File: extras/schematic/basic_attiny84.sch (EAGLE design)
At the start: 14 parts, among them U1 SI4703

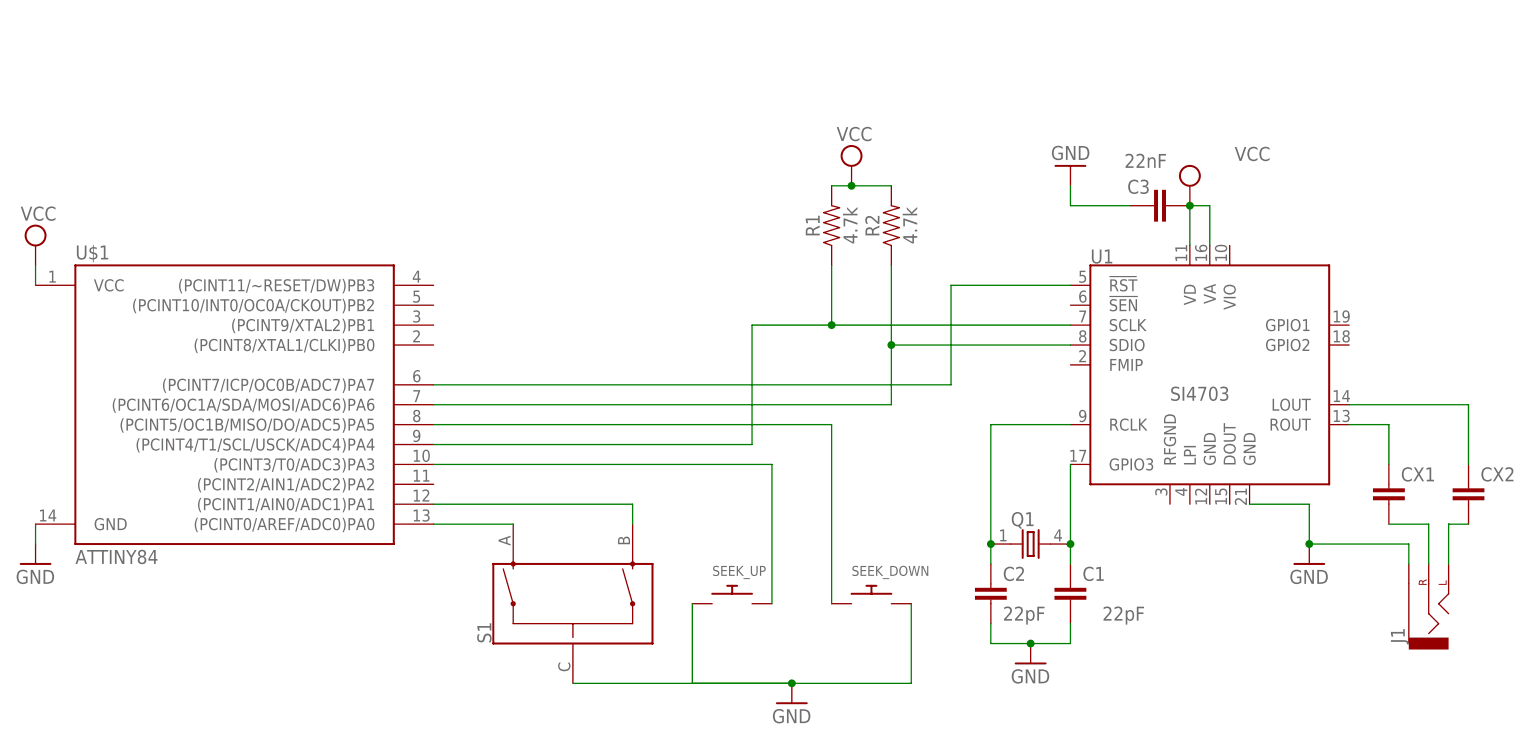
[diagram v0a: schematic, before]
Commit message: Extras
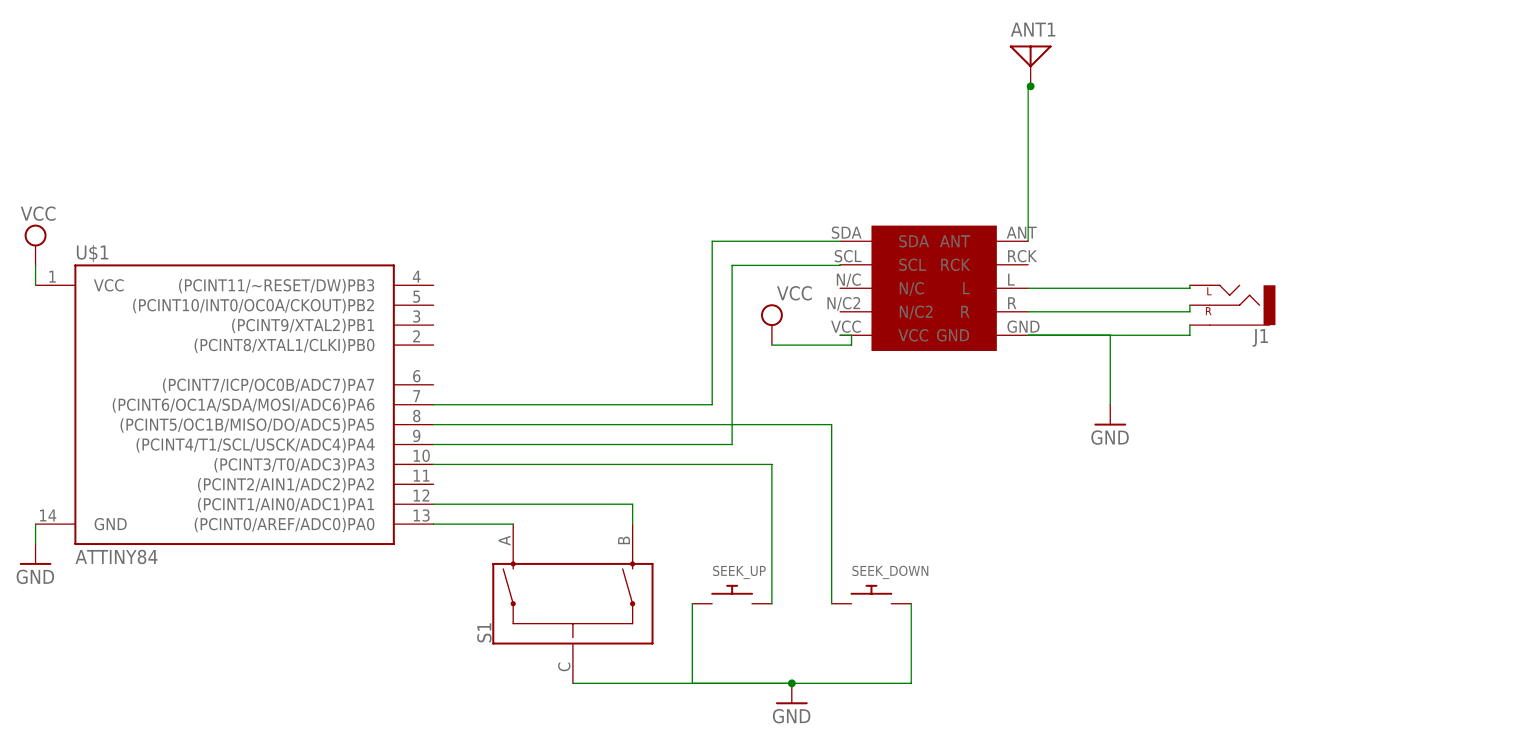
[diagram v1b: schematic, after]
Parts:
- removed C1, C2: 22pF, capacitor-wima:C2,5-3
- removed C3: 22nF, capacitor-wima:C2,5-3
- removed CX1, CX2: (no value), rcl:CXXC10B6
- removed Q1: (no value), crystal:86SMX
- removed R1, R2: 4.7k, SparkFun-Resistors:4.7KOHM-0603-1/10W-1%
- removed U1: SI4703, SI4703:SI4703
- added ANT1: (no value), discrete:ANTENNA
- added U$2: RDA, RDA:RDA
- J1: device SparkFun-Connectors:AUDIO_JACK_2.5MM_HOLESONLY -> SparkFun-Connectors:AUDIO_JACK_2.5MMSPECIAL_POGO_PINS
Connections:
- removed net N$16: CX1.1, U1.ROUT
- removed net N$19: CX2.1, U1.LOUT
- removed net N$20: CX1.2, J1.RIGHT
- removed net N$21: CX2.2, J1.LEFT
- net GND: now also U$2.GND; no longer C1.2, C2.2, C3.1, U1.GND@PAD
- net N$1: now also U$1.(PCINT6/OC1A/SDA/MOSI/ADC6)PA6, U$2.SDA; no longer R1.1, U$1.(PCINT4/T1/SCL/USCK/ADC4)PA4, U1.SCLK
- net N$2: now also U$1.(PCINT4/T1/SCL/USCK/ADC4)PA4, U$2.SCL; no longer R2.1, U$1.(PCINT6/OC1A/SDA/MOSI/ADC6)PA6, U1.SDIO
- net N$3: now also J1.LEFT, U$2.L; no longer U$1.(PCINT7/ICP/OC0B/ADC7)PA7, U1.!RST
- net N$4: now also J1.RIGHT, U$2.R; no longer C1.1, Q1.2, U1.GPIO3
- net N$5: now also ANT1.1, U$2.ANT; no longer C2.1, Q1.1, U1.RCLK
- net VCC: now also U$2.VCC; no longer C3.2, R1.2, R2.2, U1.VA, U1.VD
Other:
- moved on the sheet: J1
